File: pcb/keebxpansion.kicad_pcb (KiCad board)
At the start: 2 copper layers, 98.3 x 78.6 mm, 114 parts, among them SW1 SW_Push

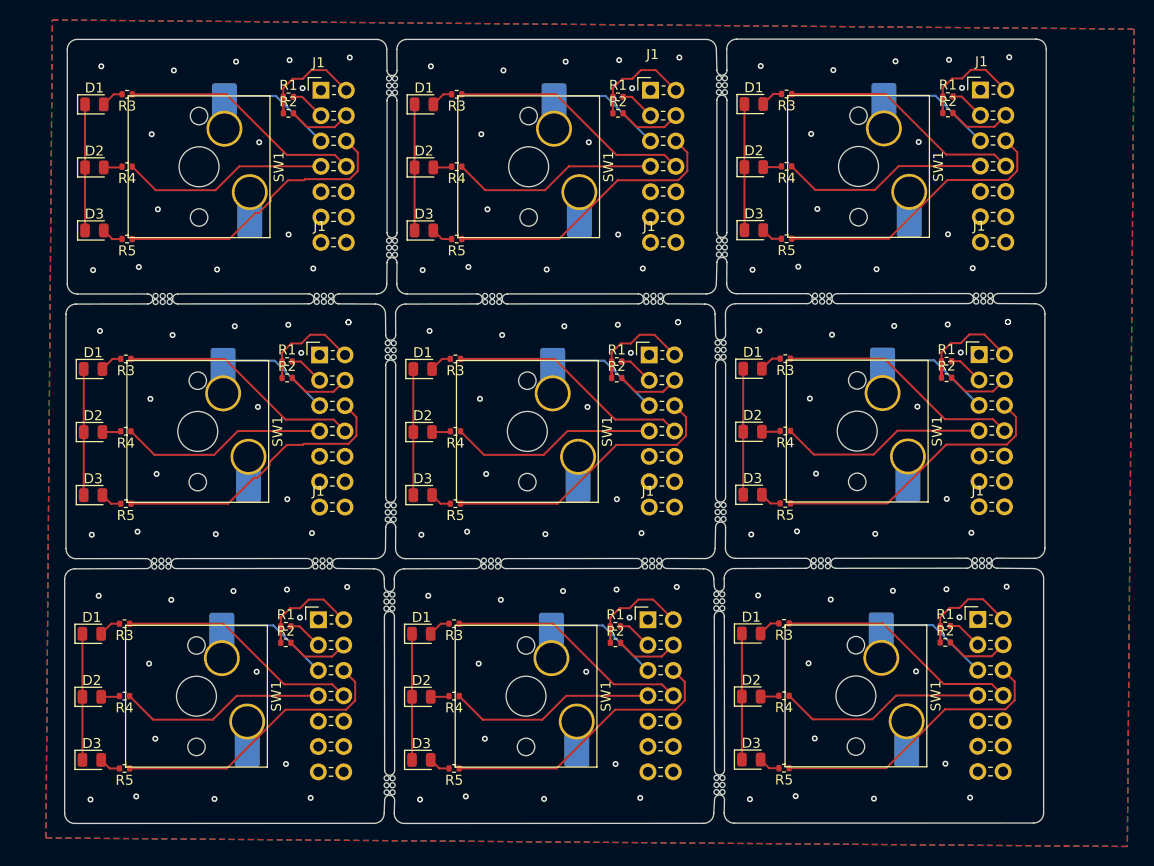
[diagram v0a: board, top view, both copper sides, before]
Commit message: pcbs 3d case and readme
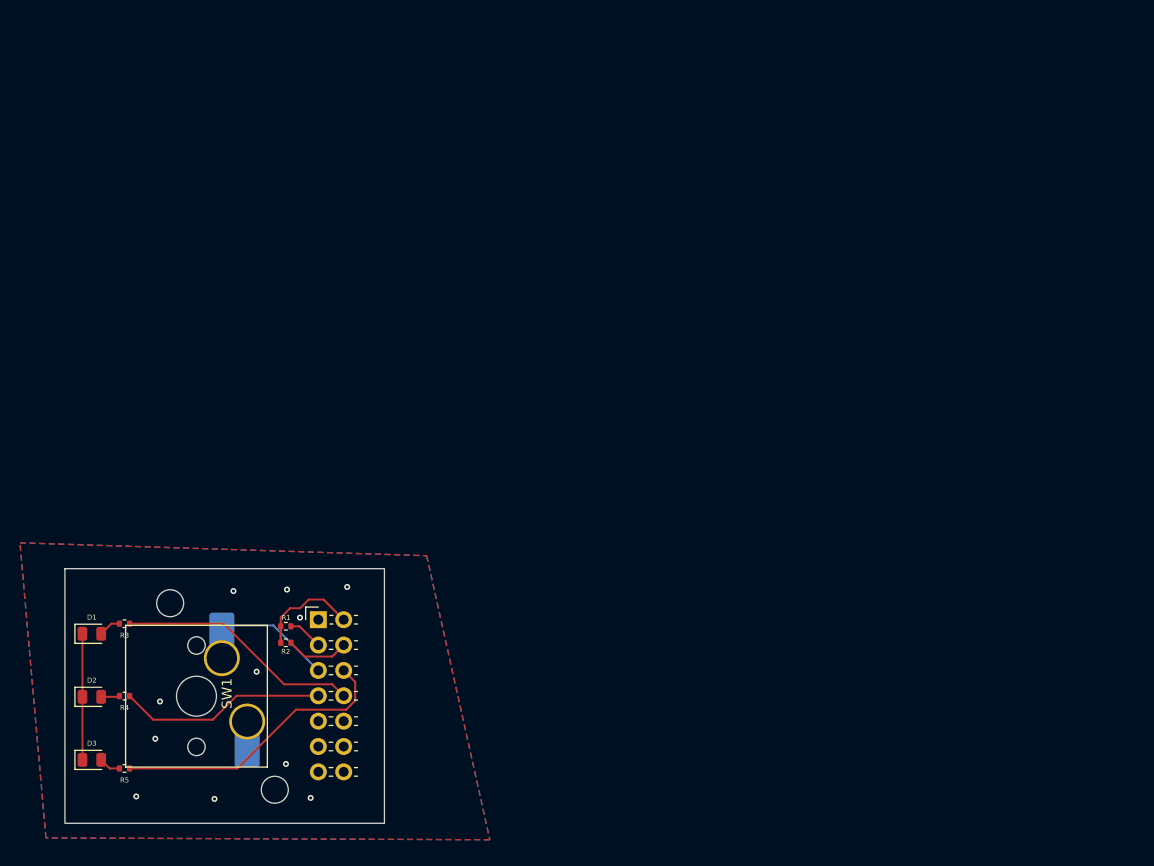
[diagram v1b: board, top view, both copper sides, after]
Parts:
- removed the D1 at (267.7, 95.5)
- removed the D1 at (267.9, 69.0)
- removed the D1 at (268.0, 42.5)
- removed the D1 at (201.8, 69.0)
- removed the D1 at (234.8, 69.0)
- removed the D1 at (235.0, 42.5)
- removed the D1 at (234.7, 95.5)
- removed the D1 at (201.9, 42.5)
- removed the D2 at (201.8, 75.3)
- removed the D2 at (267.7, 101.8)
- removed the D2 at (234.7, 101.8)
- removed the D2 at (201.9, 48.8)
- removed the D2 at (268.0, 48.8)
- removed the D2 at (235.0, 48.8)
- removed the D2 at (234.8, 75.3)
- removed the D2 at (267.9, 75.3)
- removed the D3 at (235.0, 55.1)
- removed the D3 at (268.0, 55.1)
- removed the D3 at (267.9, 81.6)
- removed the D3 at (234.8, 81.6)
- removed the D3 at (234.7, 108.1)
- removed the D3 at (201.9, 55.1)
- removed the D3 at (201.8, 81.6)
- removed the D3 at (267.7, 108.1)
- removed the J1 at (224.6, 41.1)
- removed the J1 at (257.6, 41.1)
- removed the J1 at (224.5, 67.6)
- removed the J1 at (257.5, 67.6)
- removed the J1 at (290.4, 94.1)
- removed the J1 at (257.4, 94.1)
- removed the J1 at (290.6, 67.5)
- removed the J1 at (290.7, 41.0)
- removed the R1 at (287.2, 94.7)
- removed the R1 at (254.3, 68.2)
- removed the R1 at (221.4, 41.7)
- removed the R1 at (254.4, 41.7)
- removed the R1 at (221.3, 68.2)
- removed the R1 at (254.1, 94.8)
- removed the R1 at (287.4, 41.7)
- removed the R1 at (287.3, 68.2)
- removed the R2 at (254.1, 96.4)
- removed the R2 at (254.4, 43.4)
- removed the R2 at (221.3, 69.9)
- removed the R2 at (287.4, 43.4)
- removed the R2 at (221.4, 43.4)
- removed the R2 at (287.3, 69.9)
- removed the R2 at (287.2, 96.4)
- removed the R2 at (254.3, 69.9)
- removed the R3 at (271.1, 68.0)
- removed the R3 at (271.0, 94.5)
- removed the R3 at (238.2, 41.5)
- removed the R3 at (205.1, 68.0)
- removed the R3 at (238.1, 68.0)
- removed the R3 at (205.2, 41.5)
- removed the R3 at (271.3, 41.4)
- removed the R3 at (238.0, 94.5)
- removed the R4 at (271.1, 75.2)
- removed the R4 at (238.2, 48.7)
- removed the R4 at (238.1, 75.2)
- removed the R4 at (205.2, 48.7)
- removed the R4 at (271.0, 101.7)
- removed the R4 at (205.1, 75.2)
- removed the R4 at (238.0, 101.8)
- removed the R4 at (271.3, 48.7)
- removed the R5 at (205.1, 82.5)
- removed the R5 at (271.1, 82.5)
- removed the R5 at (271.0, 109.0)
- removed the R5 at (238.0, 109.0)
- removed the R5 at (271.3, 55.9)
- removed the R5 at (238.2, 56.0)
- removed the R5 at (238.1, 82.5)
- removed the R5 at (205.2, 56.0)
- removed the SW1 at (245.3, 75.2)
- removed the SW1 at (278.4, 75.2)
- removed the SW1 at (278.2, 101.7)
- removed the SW1 at (245.2, 101.8)
- removed the SW1 at (278.5, 48.7)
- removed the SW1 at (212.3, 75.2)
- removed the SW1 at (212.4, 48.7)
- removed the SW1 at (245.4, 48.7)
- removed mouse-bite-1mm-3mm (x24): VAL**, mouse-bite:mouse-bite-1mm-3mm
- added REF**: MountingHole_2.7mm_M2.5, MountingHole:MountingHole_2.7mm_M2.5, F.Cu at (220.0, 111.1)
- added REF**: MountingHole_2.7mm_M2.5, MountingHole:MountingHole_2.7mm_M2.5, F.Cu at (209.5, 92.5)
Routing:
- net Net-(J1-GPIO1): track 260.5 -> 28.9 mm
- net Net-(J1-GPIO3): track 219.9 -> 24.4 mm
- net Net-(J1-GPI02): track 187.8 -> 20.9 mm
- net GND: track 113.7 -> 12.6 mm, vias 129 -> 11
- net +3V3: track 108.6 -> 12.1 mm
- net Net-(J1-GPIO0): track 103.8 -> 11.5 mm
- net Net-(J1-MD1): track 57.0 -> 6.33 mm
- net Net-(J1-MD0): track 31.7 -> 3.52 mm
- net Net-(D1-A): track 20.3 -> 2.25 mm
- net Net-(D3-A): track 19.7 -> 2.19 mm
- net Net-(D2-A): track 16.8 -> 1.86 mm
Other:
- board size 98.3 x 78.6 mm -> 32 x 25.5 mm
